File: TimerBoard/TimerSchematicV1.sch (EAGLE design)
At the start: 46 parts, among them IC1 STM32F10XCXT6, U2 DISPLAY-OLED-128X32, Y1 32.768kHz

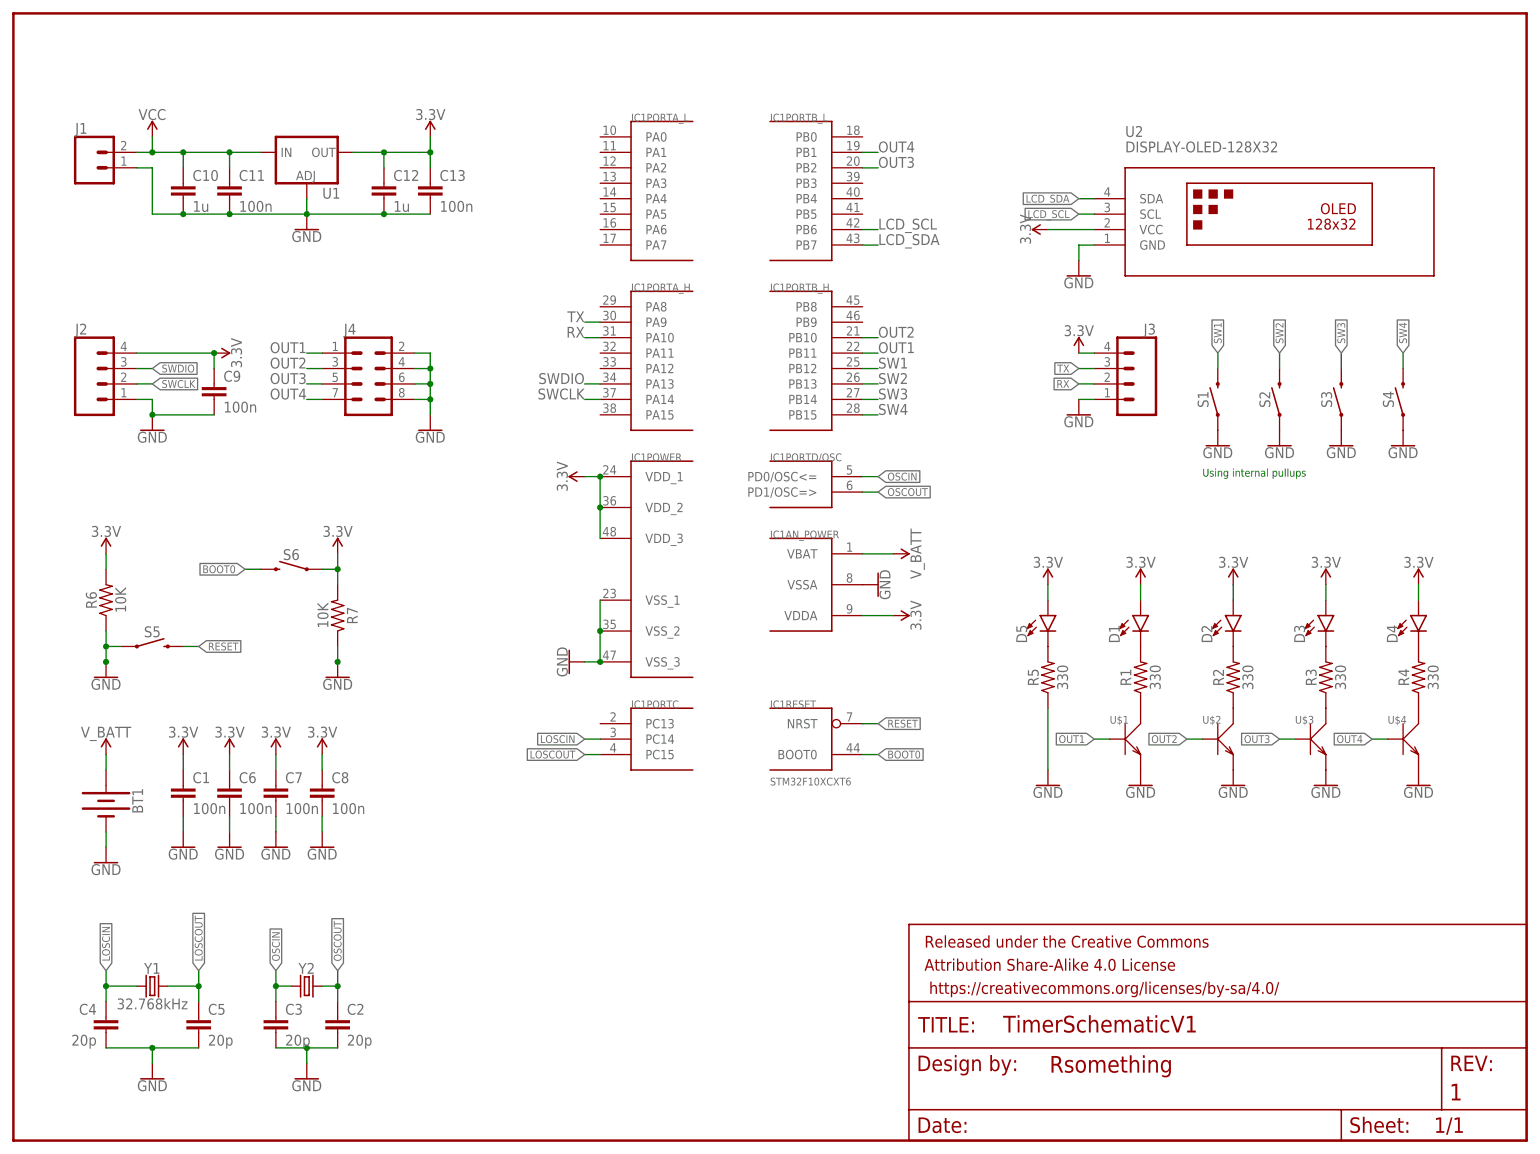
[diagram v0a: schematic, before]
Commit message: PCB alpha created
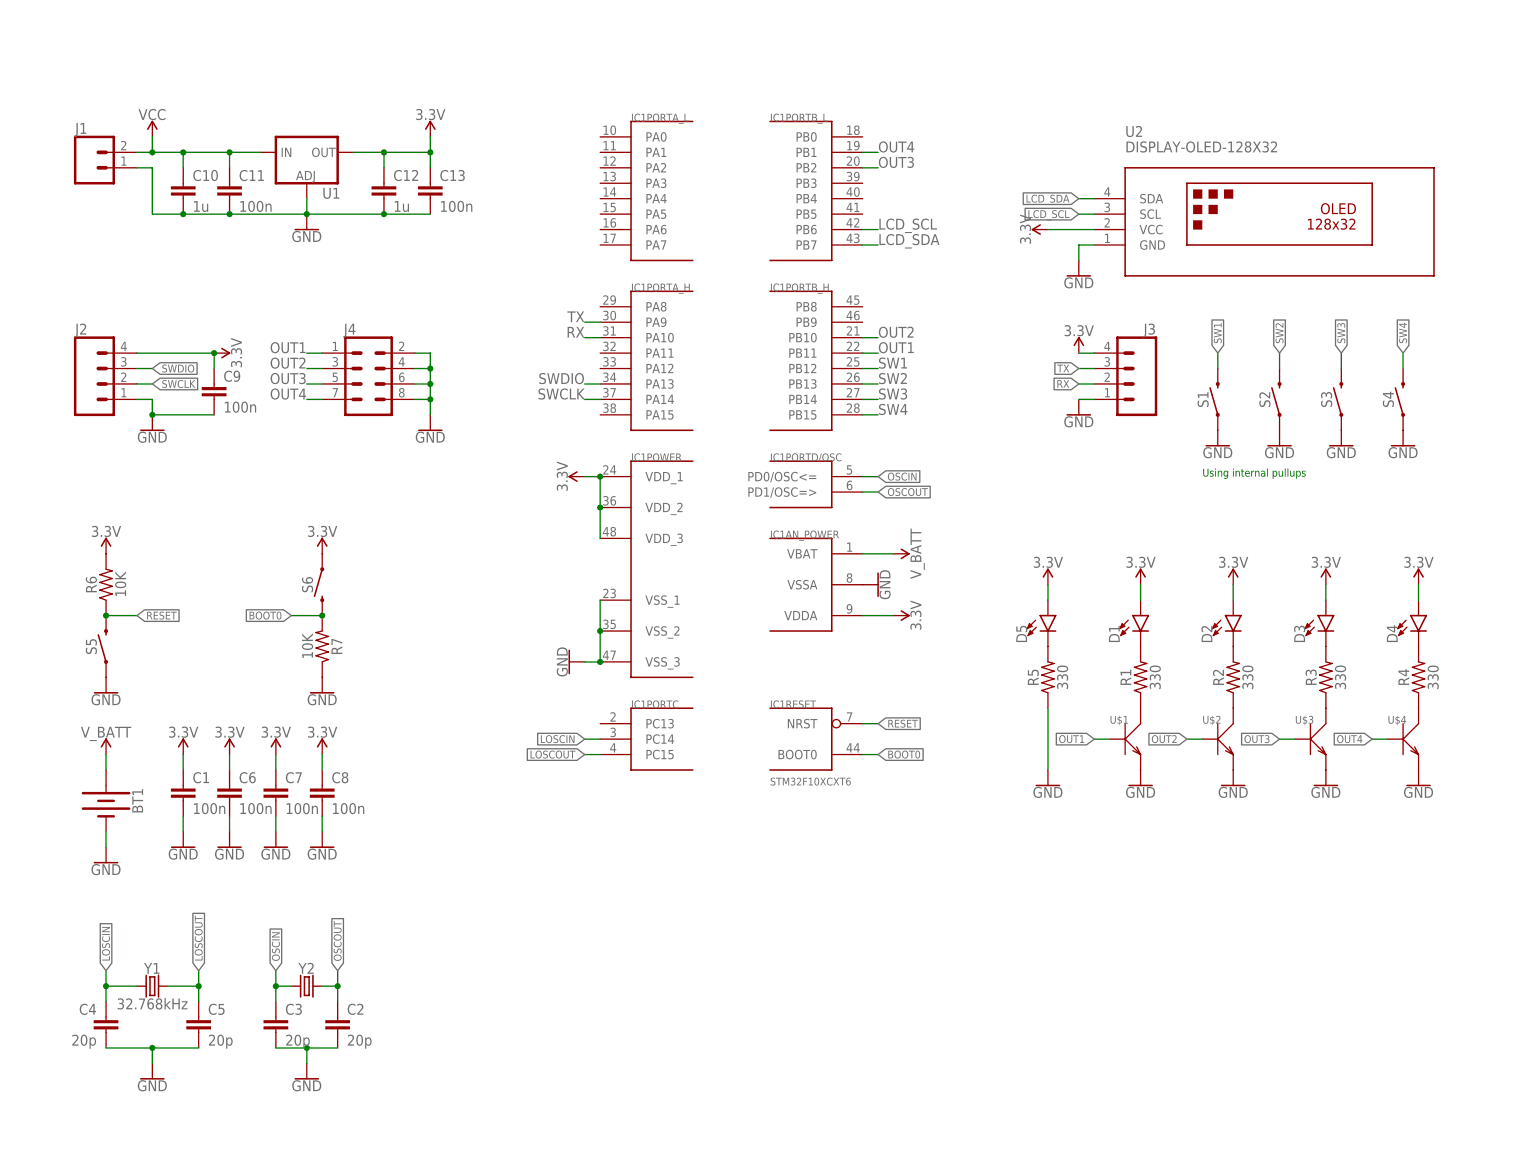
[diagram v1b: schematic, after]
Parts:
- removed FRAME1: FRAME-LETTER, SparkFun-Aesthetics:FRAME-LETTER
- J1: device SparkFun-Connectors:CONN_025MM -> SparkFun-Connectors:CONN_02
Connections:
- net 3.3V: no longer R7.2
- net BOOT0: now also R7.2
- net GND: no longer R6.1
- net RESET: now also R6.1
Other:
- moved on the sheet: R6, R7, S5, S6
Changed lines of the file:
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@@
 </groups>
 <parts>
-<part name="FRAME1" library="SparkFun-Aesthetics" deviceset="FRAME-LETTER" device="">
-<attribute name="DESIGNER" value="Rsomething"/>
-<attribute name="REV" value="1"/>
-</part>
 <part name="IC1" library="stm32" deviceset="STM32F10XCXT6" device=""/>
 <part name="U1" library="SparkFun-IC-Power" deviceset="V_REG_LM1117" device="SOT223"/>
 <part name="SUPPLY1" library="SparkFun-PowerSymbols" deviceset="3.3V" device=""/>
 <part name="SUPPLY2" library="SparkFun-PowerSymbols" deviceset="VCC" device=""/>
-<part name="J1" library="SparkFun-Connectors" deviceset="CONN_02" device="5MM"/>
+<part name="J1" library="SparkFun-Connectors" deviceset="CONN_02" device=""/>
 <part name="GND2" library="SparkFun-PowerSymbols" deviceset="GND" device=""/>
 <part name="D1" library="SparkFun-LED" deviceset="LED" device="1206"/>
@@
 <part name="GND25" library="SparkFun-PowerSymbols" deviceset="GND" device=""/>
 <part name="SUPPLY20" library="SparkFun-PowerSymbols" deviceset="3.3V" device=""/>
+<part name="FRAME1" library="SparkFun-Aesthetics" deviceset="FRAME-A4L" device=""/>
 </parts>
 <sheets>
@@
 </plain>
 <instances>
-<instance part="FRAME1" gate="G$1" x="0" y="0" smashed="yes"/>
-<instance part="FRAME1" gate="V" x="147.32" y="0" smashed="yes">
-<attribute name="LAST_DATE_TIME" x="160.02" y="1.27" size="2.54" layer="94" font="vector"/>
-<attribute name="SHEET" x="233.68" y="1.27" size="2.54" layer="94" font="vector"/>
-<attribute name="DRAWING_NAME" x="162.814" y="17.78" size="2.7432" layer="94" font="vector"/>
-<attribute name="DESIGNER" x="170.434" y="11.176" size="2.7432" layer="94" font="vector"/>
-<attribute name="REV" x="236.22" y="6.604" size="2.7432" layer="94" font="vector"/>
-</instance>
 <instance part="IC1" gate="PORTA_L" x="104.14" y="157.48" smashed="yes">
 <attribute name="NAME" x="101.6" y="167.64" size="1.27" layer="95"/>
@@
 <attribute name="VALUE" x="35.814" y="129.54" size="1.778" layer="96" font="vector" rot="R270" align="bottom-center"/>
 </instance>
-<instance part="S5" gate="G$1" x="22.86" y="81.28" smashed="yes" grouprefs="MISC">
-<attribute name="NAME" x="22.86" y="82.804" size="1.778" layer="95" font="vector" align="bottom-center"/>
-</instance>
-<instance part="S6" gate="G$1" x="45.72" y="93.98" smashed="yes" rot="MR0" grouprefs="MISC">
-<attribute name="NAME" x="45.72" y="95.504" size="1.778" layer="95" font="vector" rot="MR0" align="bottom-center"/>
-</instance>
-<instance part="R6" gate="G$1" x="15.24" y="88.9" smashed="yes" rot="R90" grouprefs="MISC">
-<attribute name="NAME" x="13.716" y="88.9" size="1.778" layer="95" font="vector" rot="R90" align="bottom-center"/>
-<attribute name="VALUE" x="16.764" y="88.9" size="1.778" layer="96" font="vector" rot="R90" align="top-center"/>
-</instance>
-<instance part="R7" gate="G$1" x="53.34" y="86.36" smashed="yes" rot="MR90" grouprefs="MISC">
-<attribute name="NAME" x="54.864" y="86.36" size="1.778" layer="95" font="vector" rot="MR90" align="bottom-center"/>
-<attribute name="VALUE" x="51.816" y="86.36" size="1.778" layer="96" font="vector" rot="MR90" align="top-center"/>
+<instance part="S5" gate="G$1" x="15.24" y="81.28" smashed="yes" rot="R90" grouprefs="MISC">
+<attribute name="NAME" x="13.716" y="81.28" size="1.778" layer="95" font="vector" rot="R90" align="bottom-center"/>
+</instance>
+<instance part="S6" gate="G$1" x="50.8" y="91.44" smashed="yes" rot="MR270" grouprefs="MISC">
+<attribute name="NAME" x="49.276" y="91.44" size="1.778" layer="95" font="vector" rot="MR270" align="bottom-center"/>
+</instance>
+<instance part="R6" gate="G$1" x="15.24" y="91.44" smashed="yes" rot="R90" grouprefs="MISC">
+<attribute name="NAME" x="13.716" y="91.44" size="1.778" layer="95" font="vector" rot="R90" align="bottom-center"/>
+<attribute name="VALUE" x="16.764" y="91.44" size="1.778" layer="96" font="vector" rot="R90" align="top-center"/>
+</instance>
+<instance part="R7" gate="G$1" x="50.8" y="81.28" smashed="yes" rot="MR90" grouprefs="MISC">
+<attribute name="NAME" x="52.324" y="81.28" size="1.778" layer="95" font="vector" rot="MR90" align="bottom-center"/>
+<attribute name="VALUE" x="49.276" y="81.28" size="1.778" layer="96" font="vector" rot="MR90" align="top-center"/>
 </instance>
 <instance part="SUPPLY10" gate="G$1" x="15.24" y="96.52" smashed="yes" grouprefs="MISC">
 <attribute name="VALUE" x="15.24" y="99.314" size="1.778" layer="96" font="vector" align="bottom-center"/>
 </instance>
-<instance part="SUPPLY11" gate="G$1" x="53.34" y="96.52" smashed="yes" rot="MR0" grouprefs="MISC">
-<attribute name="VALUE" x="53.34" y="99.314" size="1.778" layer="96" font="vector" rot="MR0" align="bottom-center"/>
-</instance>
-<instance part="GND15" gate="1" x="15.24" y="76.2" smashed="yes" grouprefs="MISC">
-<attribute name="VALUE" x="15.24" y="75.946" size="1.778" layer="96" font="vector" align="top-center"/>
-</instance>
-<instance part="GND16" gate="1" x="53.34" y="76.2" smashed="yes" rot="MR0" grouprefs="MISC">
-<attribute name="VALUE" x="53.34" y="75.946" size="1.778" layer="96" font="vector" rot="MR0" align="top-center"/>
+<instance part="SUPPLY11" gate="G$1" x="50.8" y="96.52" smashed="yes" rot="MR0" grouprefs="MISC">
+<attribute name="VALUE" x="50.8" y="99.314" size="1.778" layer="96" font="vector" rot="MR0" align="bottom-center"/>
+</instance>
+<instance part="GND15" gate="1" x="15.24" y="73.66" smashed="yes" grouprefs="MISC">
+<attribute name="VALUE" x="15.24" y="73.406" size="1.778" layer="96" font="vector" align="top-center"/>
+</instance>
+<instance part="GND16" gate="1" x="50.8" y="73.66" smashed="yes" rot="MR0" grouprefs="MISC">
+<attribute name="VALUE" x="50.8" y="73.406" size="1.778" layer="96" font="vector" rot="MR0" align="top-center"/>
 </instance>
 <instance part="BT1" gate="G$1" x="15.24" y="55.88" smashed="yes" rot="R270" grouprefs="MISC">
@@
 <instance part="SUPPLY20" gate="G$1" x="175.26" y="129.54" smashed="yes">
 <attribute name="VALUE" x="175.26" y="132.334" size="1.778" layer="96" font="vector" align="bottom-center"/>
+</instance>
+<instance part="FRAME1" gate="G$1" x="0" y="0" smashed="yes">
+<attribute name="DRAWING_NAME" x="181.61" y="11.43" size="2.54" layer="94" font="vector"/>
+<attribute name="LAST_DATE_TIME" x="181.61" y="6.35" size="2.286" layer="94" font="vector"/>
+<attribute name="SHEET" x="195.58" y="1.27" size="2.54" layer="94" font="vector"/>
+<attribute name="DESIGNER" x="226.26" y="6.35" size="2.54" layer="94" font="vector"/>
 </instance>
 </instances>
@@
 </segment>
 <segment>
-<pinref part="GND15" gate="1" pin="GND"/>
-<pinref part="R6" gate="G$1" pin="1"/>
-<wire x1="15.24" y1="78.74" x2="15.24" y2="81.28" width="0.1524" layer="91" grouprefs="MISC"/>
-<junction x="15.24" y="78.74" grouprefs="MISC"/>
-<pinref part="S5" gate="G$1" pin="1"/>
-<wire x1="15.24" y1="81.28" x2="15.24" y2="83.82" width="0.1524" layer="91" grouprefs="MISC"/>
-<wire x1="17.78" y1="81.28" x2="15.24" y2="81.28" width="0.1524" layer="91" grouprefs="MISC"/>
-<junction x="15.24" y="81.28" grouprefs="MISC"/>
-</segment>
-<segment>
-<pinref part="GND16" gate="1" pin="GND"/>
-<pinref part="R7" gate="G$1" pin="1"/>
-<wire x1="53.34" y1="81.28" x2="53.34" y2="78.74" width="0.1524" layer="91" grouprefs="MISC"/>
-<junction x="53.34" y="78.74" grouprefs="MISC"/>
-</segment>
-<segment>
 <pinref part="BT1" gate="G$1" pin="-"/>
 <pinref part="GND17" gate="1" pin="GND"/>
@@
 <junction x="68.58" y="127" grouprefs="HEADERS"/>
 </segment>
+<segment>
+<pinref part="GND16" gate="1" pin="GND"/>
+<pinref part="R7" gate="G$1" pin="1"/>
+</segment>
+<segment>
+<pinref part="GND15" gate="1" pin="GND"/>
+<pinref part="S5" gate="G$1" pin="1"/>
+</segment>
 </net>
 <net name="3.3V" class="0">
@@
 </segment>
 <segment>
-<pinref part="SUPPLY10" gate="G$1" pin="3.3V"/>
-<pinref part="R6" gate="G$1" pin="2"/>
-<wire x1="15.24" y1="96.52" x2="15.24" y2="93.98" width="0.1524" layer="91" grouprefs="MISC"/>
-</segment>
-<segment>
-<pinref part="SUPPLY11" gate="G$1" pin="3.3V"/>
-<pinref part="R7" gate="G$1" pin="2"/>
-<wire x1="53.34" y1="96.52" x2="53.34" y2="93.98" width="0.1524" layer="91" grouprefs="MISC"/>
-<pinref part="S6" gate="G$1" pin="1"/>
-<wire x1="53.34" y1="93.98" x2="53.34" y2="91.44" width="0.1524" layer="91" grouprefs="MISC"/>
-<wire x1="50.8" y1="93.98" x2="53.34" y2="93.98" width="0.1524" layer="91" grouprefs="MISC"/>
-<junction x="53.34" y="93.98" grouprefs="MISC"/>
-</segment>
-<segment>
 <pinref part="SUPPLY14" gate="G$1" pin="3.3V"/>
 <pinref part="C1" gate="G$1" pin="1"/>
@@
 <pinref part="SUPPLY20" gate="G$1" pin="3.3V"/>
 </segment>
+<segment>
+<pinref part="S6" gate="G$1" pin="1"/>
+<pinref part="SUPPLY11" gate="G$1" pin="3.3V"/>
+</segment>
+<segment>
+<pinref part="SUPPLY10" gate="G$1" pin="3.3V"/>
+<pinref part="R6" gate="G$1" pin="2"/>
+</segment>
 </net>
 <net name="N$1" class="0">
@@
 <segment>
 <pinref part="S5" gate="G$1" pin="2"/>
-<wire x1="27.94" y1="81.28" x2="30.48" y2="81.28" width="0.1524" layer="91" grouprefs="MISC"/>
-<label x="30.48" y="81.28" size="1.27" layer="95" xref="yes" grouprefs="MISC"/>
+<wire x1="15.24" y1="86.36" x2="20.32" y2="86.36" width="0.1524" layer="91" grouprefs="MISC"/>
+<label x="20.32" y="86.36" size="1.27" layer="95" xref="yes" grouprefs="MISC"/>
+<pinref part="R6" gate="G$1" pin="1"/>
+<junction x="15.24" y="86.36"/>
 </segment>
 <segment>
@@
 <segment>
 <pinref part="S6" gate="G$1" pin="2"/>
-<wire x1="40.64" y1="93.98" x2="38.1" y2="93.98" width="0.1524" layer="91" grouprefs="MISC"/>
-<label x="38.1" y="93.98" size="1.27" layer="95" rot="MR0" xref="yes" grouprefs="MISC"/>
-</segment>
-<segment>
+<wire x1="50.8" y1="86.36" x2="45.72" y2="86.36" width="0.1524" layer="91" grouprefs="MISC"/>
+<label x="45.72" y="86.36" size="1.27" layer="95" rot="MR0" xref="yes" grouprefs="MISC"/>
+<pinref part="R7" gate="G$1" pin="2"/>
+<junction x="50.8" y="86.36"/>
+</segment>
+<segment>
